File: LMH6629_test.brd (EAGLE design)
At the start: 50 x 50 mm, 20 parts, among them X1 1-227161-0, X2 SMA-142-0711-871/876

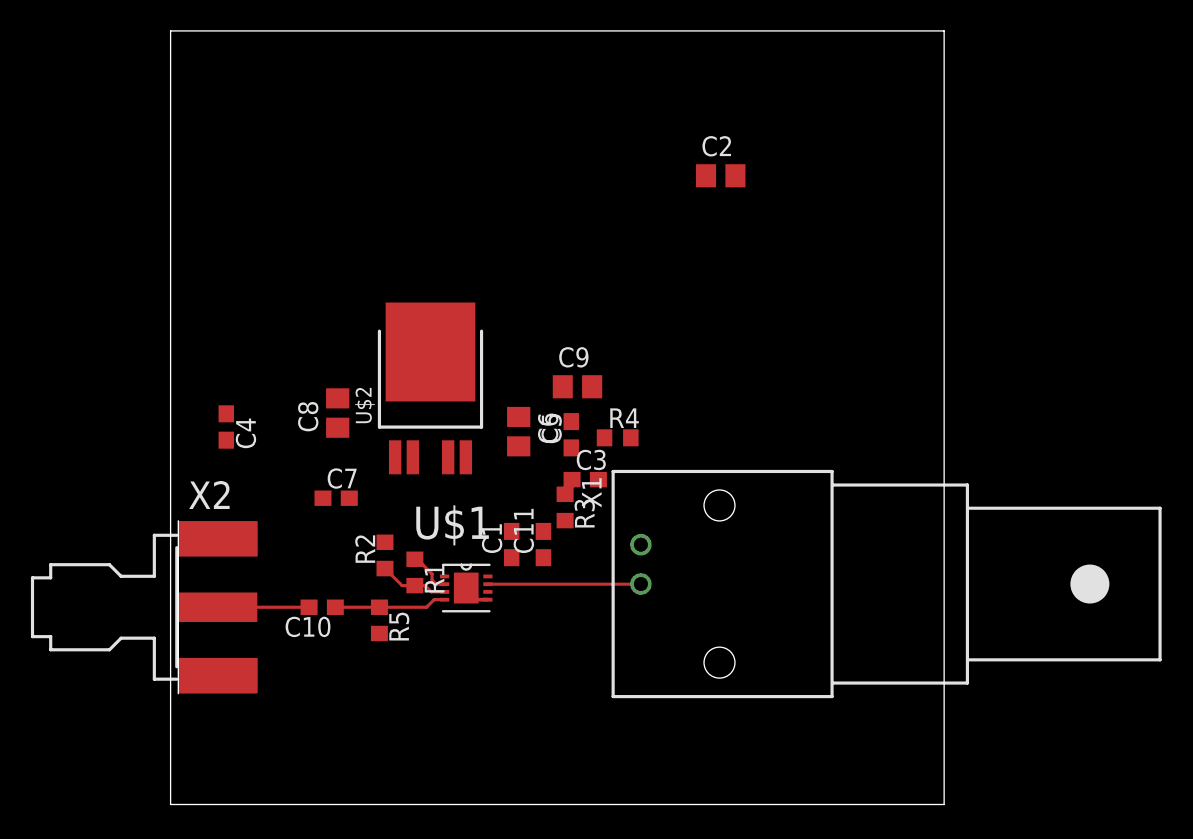
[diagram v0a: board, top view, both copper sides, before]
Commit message: some progress on pcb
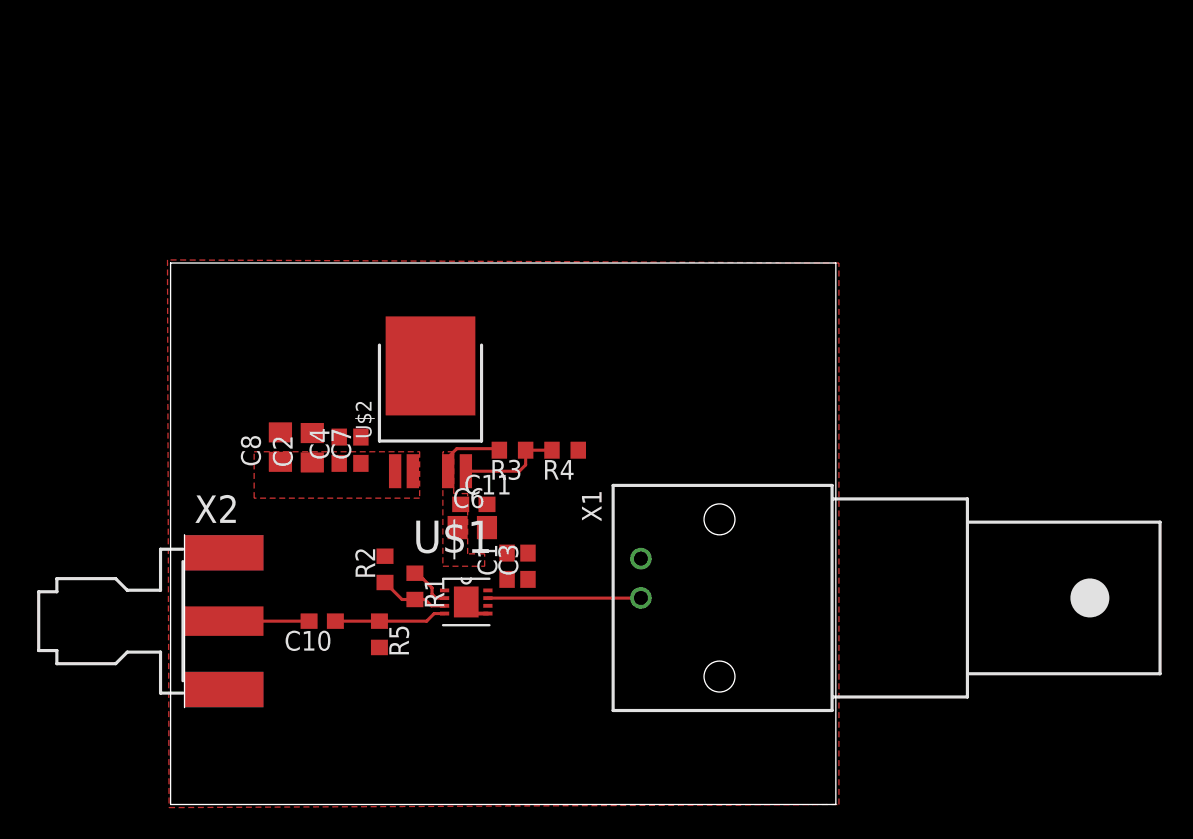
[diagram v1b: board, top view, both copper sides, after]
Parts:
- removed C5: (no value), rcl:C0603
- removed C9: (no value), rcl:C0805
- moved C2 31.7 mm to (9.16, 23.1), turned to 90 degrees
- moved C4 7.45 mm to (10.9, 22.9), turned to 90 degrees
- moved C6 6.89 mm to (19.5, 17.9), turned to 0 degrees
- moved C3 6.71 mm to (23.1, 15.4), turned to 90 degrees
- moved C11 5.20 mm to (19.6, 19.4), turned to 0 degrees
- moved R3 5.02 mm to (22.1, 22.9), turned to 180 degrees
- moved C8 4.30 mm to (7.10, 23.1)
- moved R4 3.49 mm to (25.5, 22.9), turned to 180 degrees
- moved C7 3.49 mm to (12.3, 22.9), turned to 90 degrees
- moved C1 1.43 mm to (21.8, 15.4)
- moved X2 0.98 mm to (0.90, 11.8)
- moved R2 0.90 mm to (13.9, 15.2)
- moved U$2 0.90 mm to (16.8, 28.4)
- moved C10 0.90 mm to (9.80, 11.8)
- moved R1 0.90 mm to (15.8, 14.1)
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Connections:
- net N$4 renamed ADJ
- net GND: no longer C5.2, C9.2
- net V_ANALOG: no longer C5.1, C9.1
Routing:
- net ADJ: track 0.00 -> 6.68 mm
- net V_ANALOG: track 0.00 -> 4.48 mm
- added copper zone on layer 1, net GND
- added copper zone on layer 1, net PWR_IN
- added copper zone on layer 1, net V_ANALOG
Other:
- board size 50 x 50 mm -> 43 x 35 mm
